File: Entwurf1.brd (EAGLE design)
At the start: 91.4 x 101.6 mm, 5 parts, among them X2 DTF13-12PA

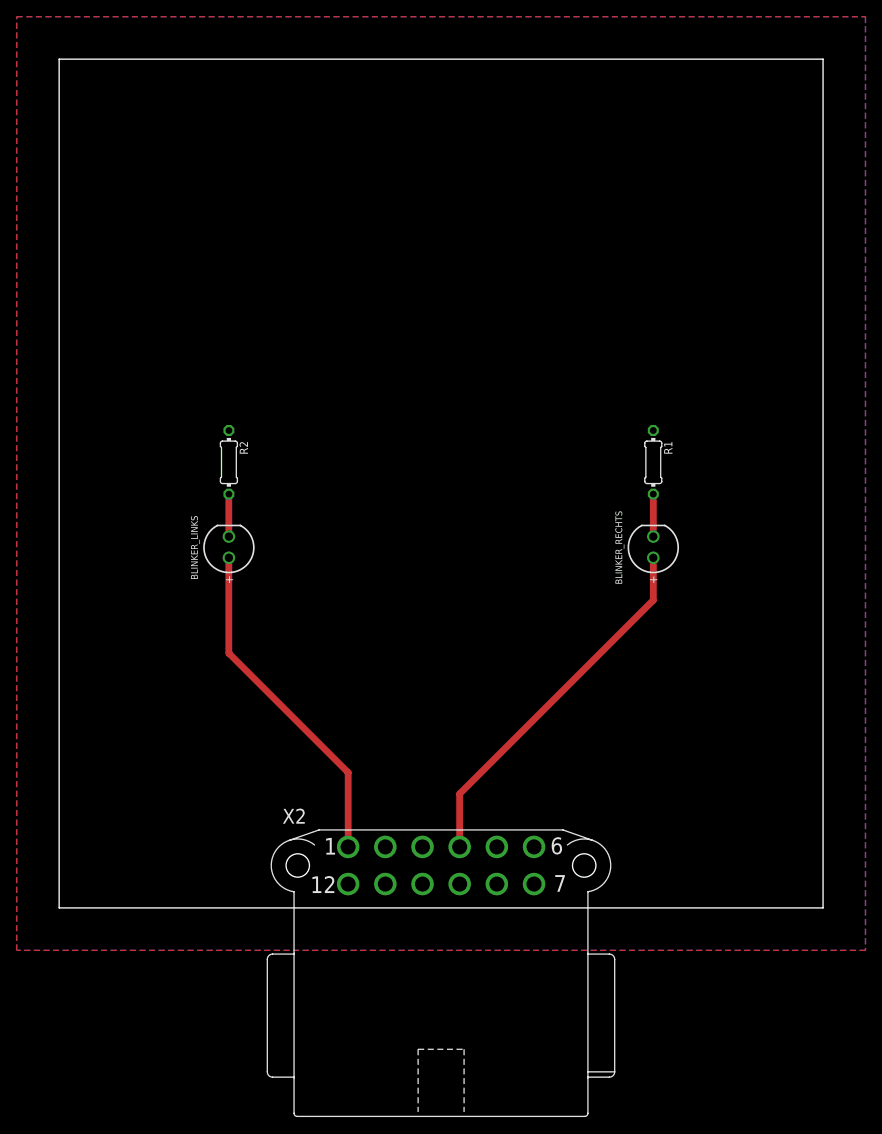
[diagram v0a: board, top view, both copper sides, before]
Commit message: ..
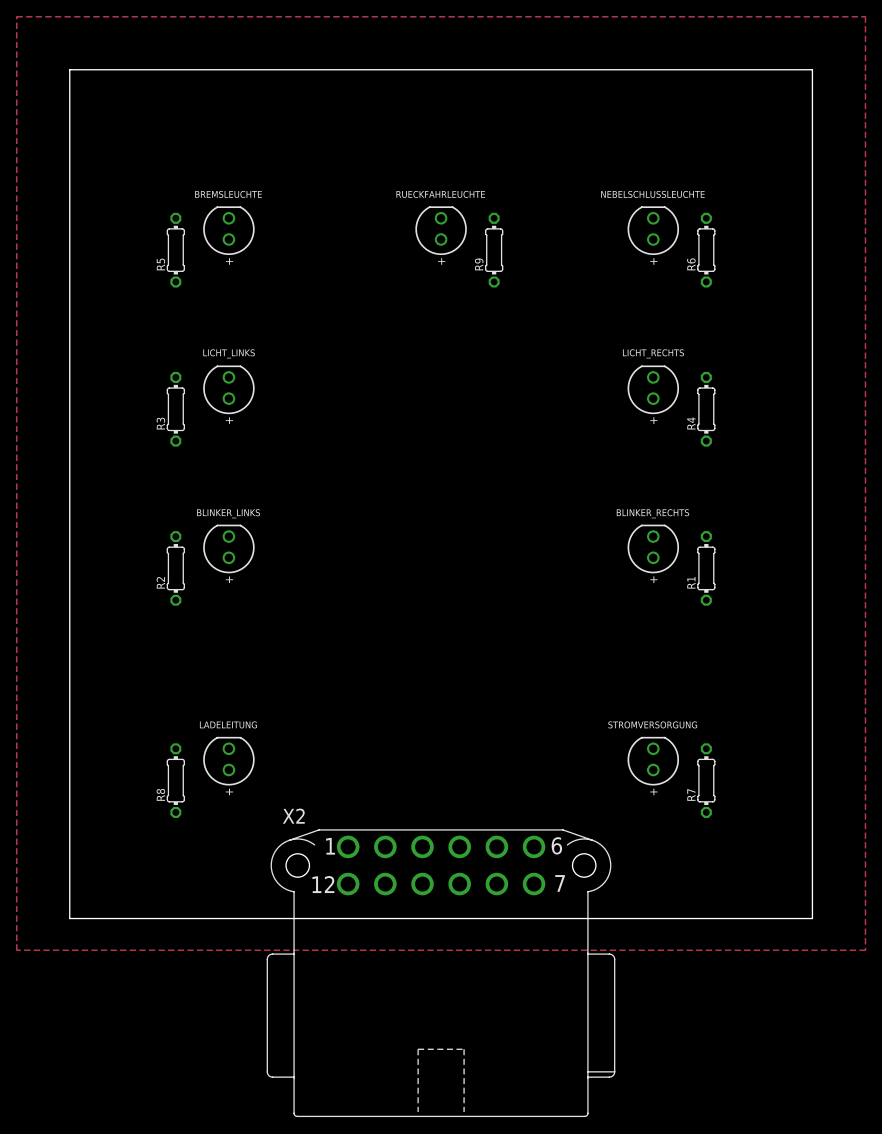
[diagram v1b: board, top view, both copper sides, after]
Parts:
- added BREMSLEUCHTE, LICHT_LINKS, LICHT_RECHTS: Rot, Wurth_LEDs_WL-TMRW:WL-TMRW_5MM
- added LADELEITUNG, NEBELSCHLUSSLEUCHTE, RUECKFAHRLEUCHTE, STROMVERSORGUNG: Grün, Wurth_LEDs_WL-TMRW:WL-TMRW_5MM
- added R3, R4, R5, R6, R7, R8, R9: 680, resistor:0204/7
- moved R1 14.2 mm to (31.8, 35.6), turned to 90 degrees
- moved R2 14.2 mm to (-31.8, 35.6), turned to 90 degrees
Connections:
- net BLINKER_LINKS renamed BLINKER_LINKS_1
- net BLINKER_RECHTS renamed BLINKER_RECHTS_4
- removed net BREMSLEUCHTE: X2.6
- removed net LADELEITUNG: X2.10
- removed net LICHT_LINKS: X2.7
- removed net LICHT_RECHTS: X2.5
- removed net MASSE: R1.1, R2.1, X2.3
- removed net MASSE_9_12: X2.12
- removed net MASSE_LADELEITUNG: X2.11
- removed net NEBELSCHLUSSLEUCHTE: X2.2
- removed net RUECKFAHRLEUCHTE: X2.8
- removed net STROMVERSORGUNG: X2.9
- new net BREMSLEUCHTE_6: BREMSLEUCHTE.2, X2.6
- new net LADELEITUNG_10: LADELEITUNG.2, X2.10
- new net LICHT_LINKS_7: LICHT_LINKS.2, X2.7
- new net LICHT_RECHTS_5: LICHT_RECHTS.2, X2.5
- new net MASSE_1_8: R1.1, R2.1, R3.1, R4.1, R5.1, R6.1, R9.1, X2.3
- new net MASSE_9: R7.1, R8.1, X2.12
- new net N$1: LICHT_LINKS.1, R3.2
- new net N$2: LICHT_RECHTS.1, R4.2
- new net N$4: BREMSLEUCHTE.1, R5.2
- new net N$6: NEBELSCHLUSSLEUCHTE.1, R6.2
- new net N$7: R7.2, STROMVERSORGUNG.1
- new net N$8: LADELEITUNG.1, R8.2
- new net N$9: R9.2, RUECKFAHRLEUCHTE.1
- new net NEBELSCHLUSSLEUCHTE_2: NEBELSCHLUSSLEUCHTE.2, X2.2
- new net RUECKFAHRLEUCHTE_8: RUECKFAHRLEUCHTE.2, X2.8
- new net STROMVERSORGUNG_9: STROMVERSORGUNG.2, X2.9
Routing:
- net BLINKER_RECHTS_4: track 44.2 -> 0.00 mm
- net BLINKER_LINKS_1: track 40.5 -> 0.00 mm
- net N$5: track 5.08 -> 0.00 mm
- net N$3: track 5.08 -> 0.00 mm
- added copper zone on layer 1, net MASSE_1_8
- added copper zone on layer 16, net MASSE_1_8
- removed copper zone on layer 1, net MASSE
- removed copper zone on layer 16, net MASSE
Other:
- board size 91.4 x 101.6 mm -> 88.9 x 101.6 mm
